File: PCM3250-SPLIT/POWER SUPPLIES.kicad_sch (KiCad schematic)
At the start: 50 parts, among them IC3 TPS65133, U3 LMR51430, U8 LMR51430

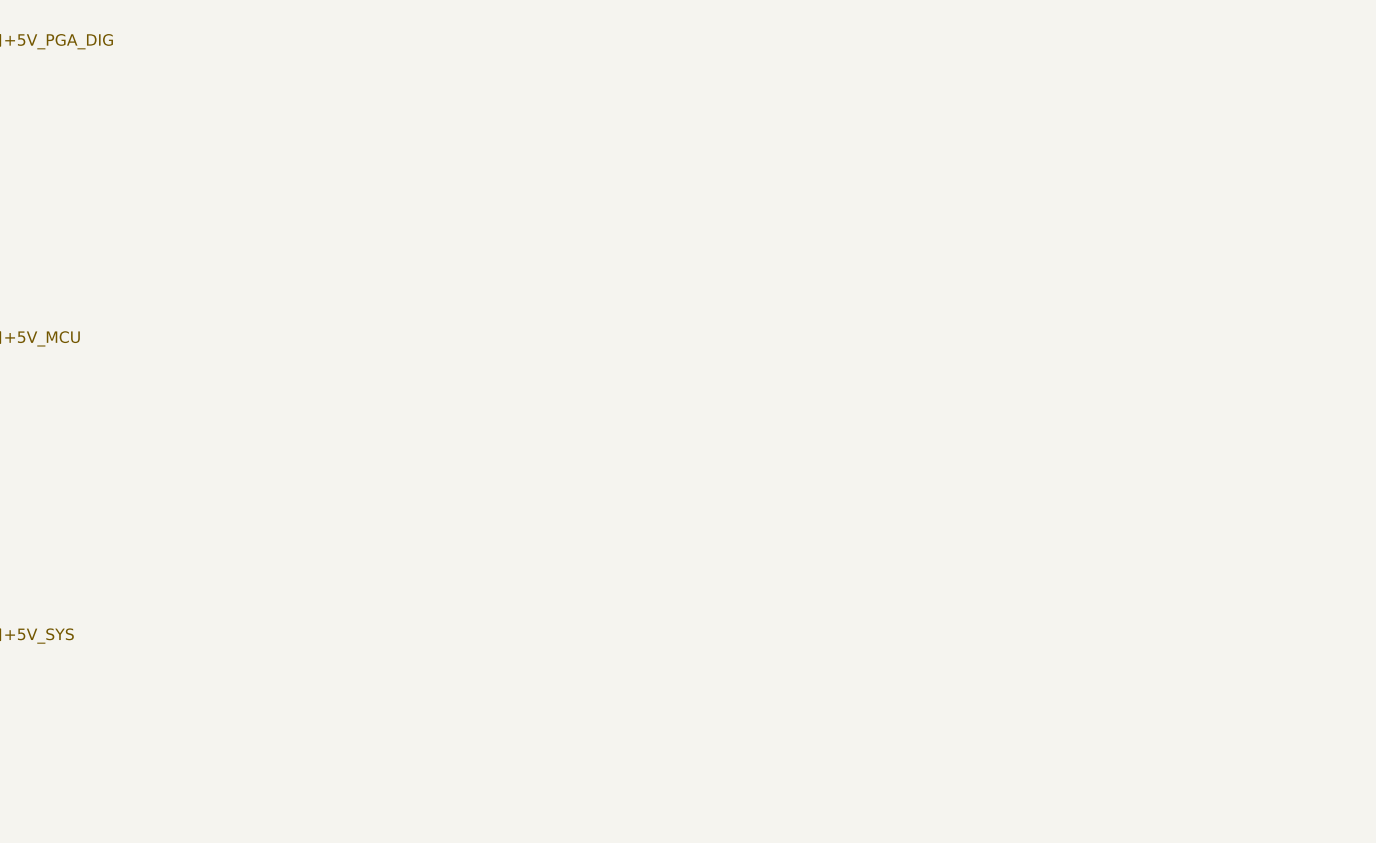
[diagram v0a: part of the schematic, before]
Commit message: lots of work
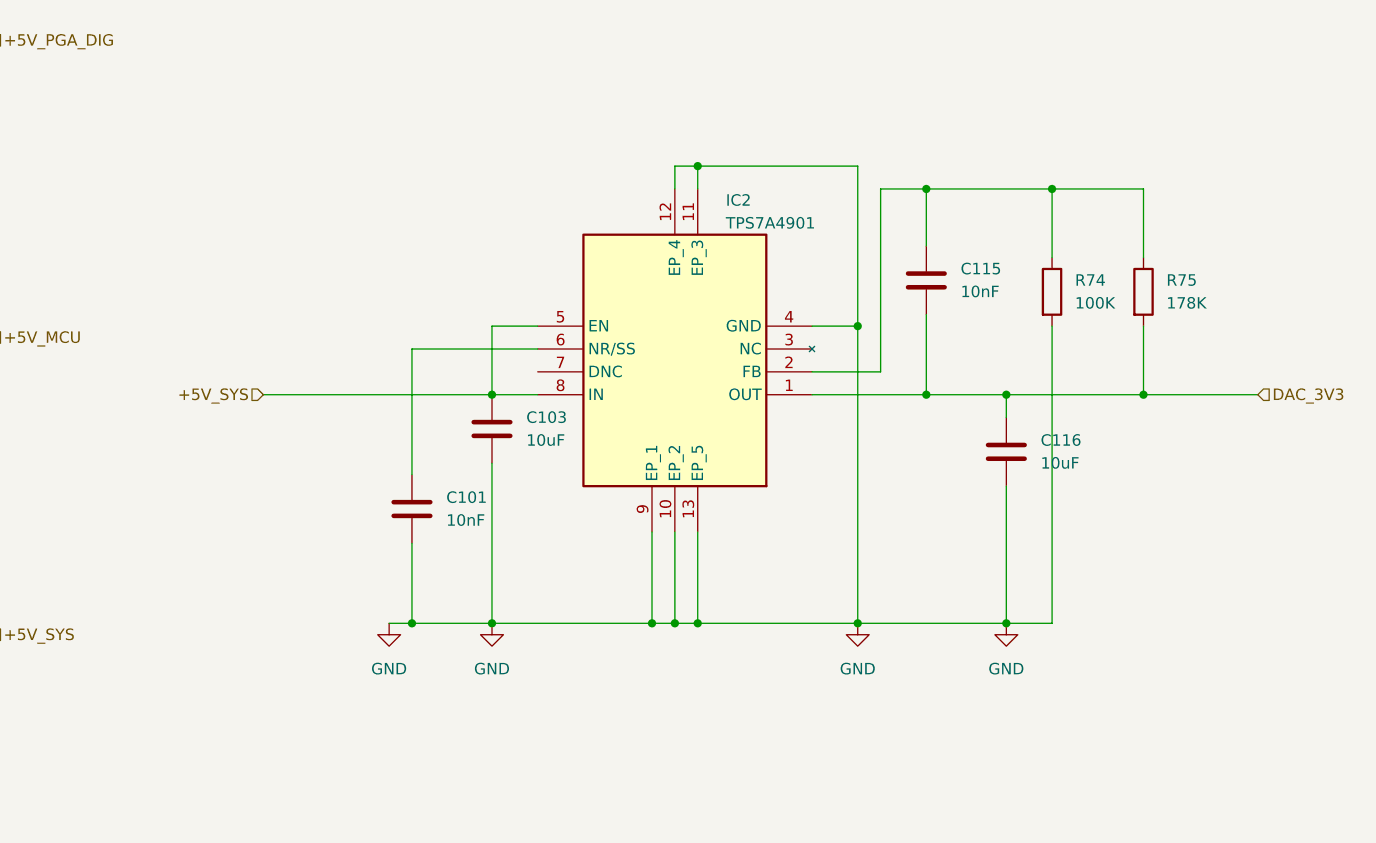
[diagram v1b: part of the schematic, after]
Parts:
- added C101, C115: 10nF, Capacitor_SMD:C_0805_2012Metric_Pad1.18x1.45mm_HandSolder, symbol Device:C
- added C103, C116: 10uF, Capacitor_SMD:C_1206_3216Metric_Pad1.33x1.80mm_HandSolder, symbol Device:C
- added IC2: TPS7A4901, Custom:TPS7A4901DRBR, symbol Custom:TPS7A4901DRBR
- added R74: 100K, Resistor_SMD:R_0805_2012Metric_Pad1.20x1.40mm_HandSolder, symbol Device:R
- added R75: 178K, Resistor_SMD:R_0805_2012Metric_Pad1.20x1.40mm_HandSolder, symbol Device:R
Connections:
- net +5V_SYS: now also C103.2, IC2.5 (EN), IC2.8 (IN)
- net GND: now also C101.2, C103.1, C116.1, IC2.10 (EP_2), IC2.11 (EP_3), IC2.12 (EP_4), IC2.13 (EP_5), IC2.4 (GND), IC2.9 (EP_1), R74.2
- new net: C101.1, IC2.6 (NR/SS)
- new net: C115.1, IC2.2 (FB), R74.1, R75.1
- new net DAC_3V3: C115.2, C116.2, IC2.1 (OUT), R75.2
